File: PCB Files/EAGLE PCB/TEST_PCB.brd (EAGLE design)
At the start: 33.6 x 25.5 mm, 22 parts, among them IC1 4066D, IC2 OP-AMP

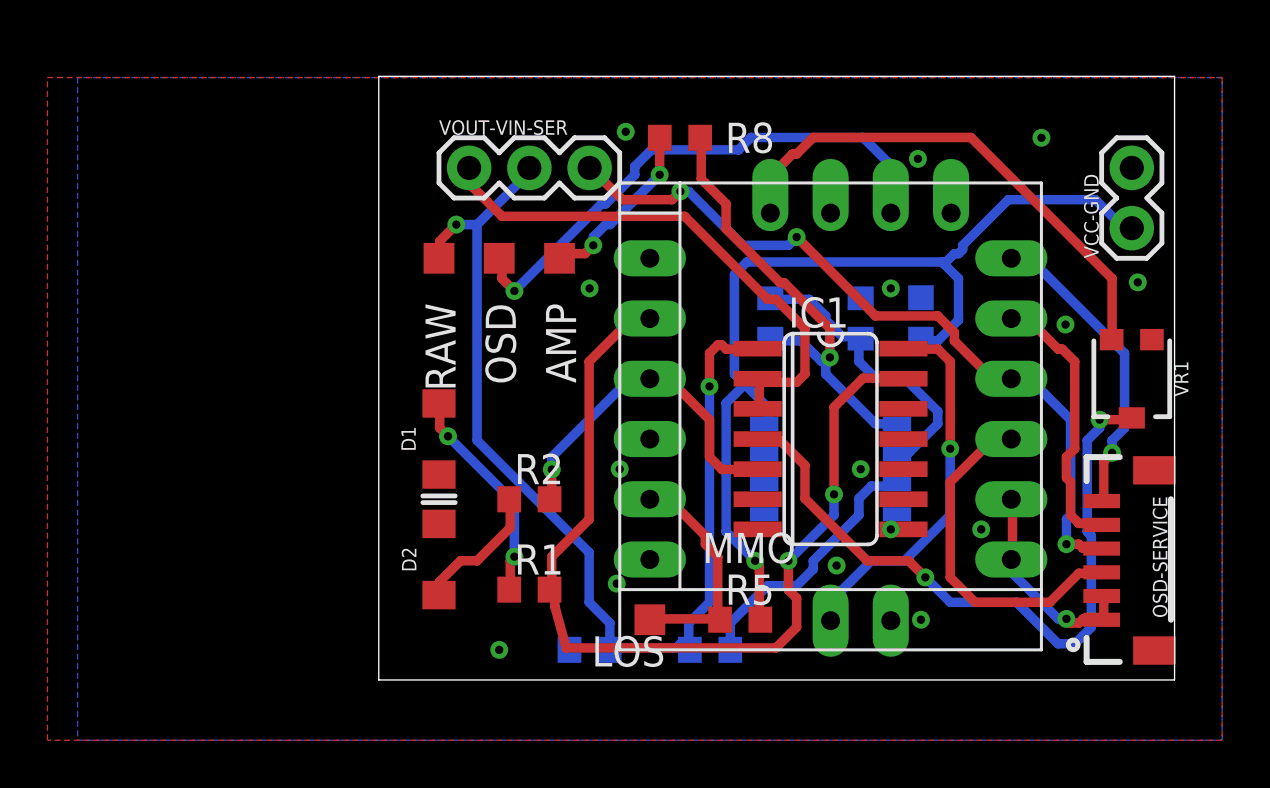
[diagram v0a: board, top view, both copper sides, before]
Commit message: Experimental PCBs
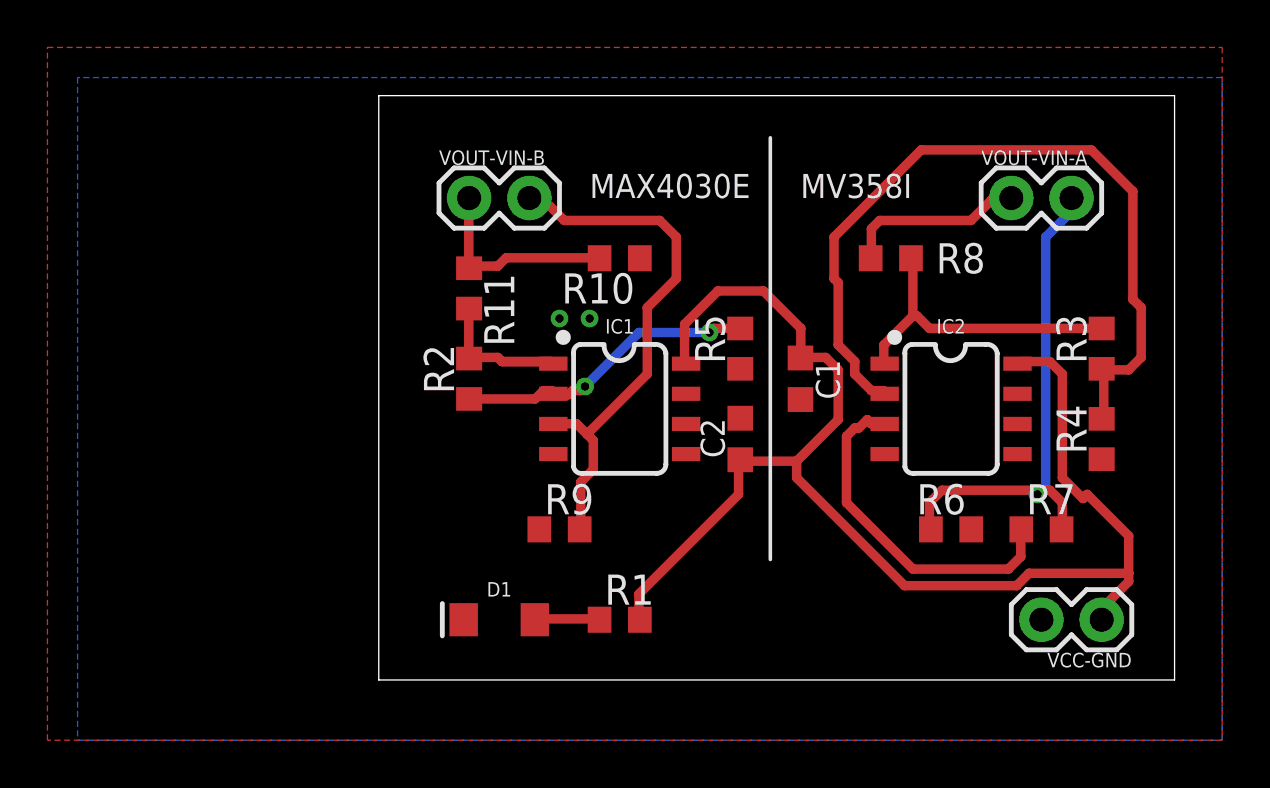
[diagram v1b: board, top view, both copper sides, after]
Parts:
- removed AMP, LOS, OSD, RAW: TPSQTP13SQ, testpad:TP13SQ
- removed D2: RED, SparkFun-LED:LED-1206
- removed MINIMOSD: MICROMINIMOSDPWR, FPVTools:MMOSDNVDVID
- removed OSD-SERVICE: EM406, SparkFun-Connectors:1X06-1MM
- removed VOUT-VIN-SER: (no value), SparkFun-Connectors:1X03
- removed VR1: 10k, SparkFun-Resistors:TRIMPOT-SMD-3MM-CLOSED
- added C2: o.1uF, rcl:C0603K
- added R10, R11, R9: 75, resistor:R0603
- added VOUT-VIN-A, VOUT-VIN-B: (no value), SparkFun-Connectors:1X02
- IC1: value 4066D -> OP-AMP; device 40xx:SO14 -> SparkFun-IC-Amplifiers:SO08
- R2: value 330 -> 200
- R5: value 1k -> 200
- moved VCC-GND 16.6 mm to (41.9, 53.3), turned to 180 degrees
- moved R6 16.1 mm to (35.6, 57.1), flipped to the top
- moved R7 14.9 mm to (39.4, 57.1), flipped to the top
- moved R3 14.0 mm to (41.9, 64.8), flipped to the top, turned to 90 degrees
- moved R5 11.4 mm to (26.7, 64.8), turned to 90 degrees
- moved R4 11.4 mm to (41.9, 61.0), flipped to the top, turned to 90 degrees
- moved R8 10.2 mm to (33.0, 68.6)
- moved IC1 8.98 mm to (21.6, 62.2)
- moved D1 8.03 mm to (16.5, 53.3), turned to 180 degrees
- moved IC2 5.68 mm to (35.6, 62.2), flipped to the top
- moved C1 5.68 mm to (29.2, 63.5), flipped to the top, turned to 270 degrees
- moved R2 5.68 mm to (15.2, 63.5), turned to 90 degrees
- moved R1 4.02 mm to (21.6, 53.3)
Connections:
- removed net 5VFTDI: MINIMOSD.VCC, OSD-SERVICE.3
- removed net AMP: AMP.TP, R8.1
- removed net BAT2: MINIMOSD.BAT2
- removed net CONTROLL_A: IC1.13, MINIMOSD.CGND, R1.2
- removed net CONTROLL_B: IC1.5, MINIMOSD.RSSI, R2.2
- removed net DTR: MINIMOSD.DTR, OSD-SERVICE.6
- removed net G: MINIMOSD.GND1, MINIMOSD.GND2, OSD-SERVICE.1, OSD-SERVICE.2
- removed net N$3: LOS.TP, MINIMOSD.BAT1, R5.1
- removed net N$6: MINIMOSD.VIDOUT, VR1.3
- removed net OSD: MINIMOSD.VIDIN, OSD.TP
- removed net OSD_OUT: IC1.4, VR1.2
- removed net RX: MINIMOSD.RX, OSD-SERVICE.4, VOUT-VIN-SER.3
- removed net TX: MINIMOSD.TX, OSD-SERVICE.5
- removed net VDD: IC1.14, MINIMOSD.IVCC
- removed net VIDEO_IN: IC1.1, R6.2, R7.2, RAW.TP, VOUT-VIN-SER.2
- removed net VIDEO_OUT: IC1.2, IC1.3, VOUT-VIN-SER.1
- removed net VSS: IC1.7
- new net 1: IC1.1, R11.2, R2.2
- new net VIDEO_IN_A: R6.2, R7.2, VOUT-VIN-A.2
- new net VIDEO_IN_B: IC1.3, R9.2, VOUT-VIN-B.2
- new net VIDEO_OUT_A: R8.1, VOUT-VIN-A.1
- new net VIDEO_OUT_B: R10.2, R11.1, VOUT-VIN-B.1
- net GND: now also C2.2, IC1.4, R10.1, R5.1, R9.1; no longer D2.C, IC1.11, IC1.8, MINIMOSD.BGND, MINIMOSD.CUR, MINIMOSD.IGND, MINIMOSD.VGND1, MINIMOSD.VGND2
- net N$1: now also IC1.2, R5.2; no longer D2.A
- net VCC: now also C2.1, IC1.8, R1.2; no longer R5.2
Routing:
- net VIDEO_IN: track 45.3 -> 0.00 mm, vias 2 -> 0
- net CONTROLL_A: track 40.3 -> 0.00 mm, vias 2 -> 0
- net RX: track 32.4 -> 0.00 mm, vias 3 -> 0
- net OSD_OUT: track 29.2 -> 0.00 mm, vias 2 -> 0
- net OSD: track 22.9 -> 0.00 mm, vias 1 -> 0
- net VIDEO_OUT: track 22.8 -> 0.00 mm
- net VIDEO_IN_B: track 0.00 -> 22.7 mm
- net N$6: track 21.7 -> 0.00 mm
- net VIDEO_IN_A: track 0.00 -> 21.7 mm, vias 0 -> 1
- net N$4: track 12.6 -> 34.0 mm
- net VCC: track 41.2 -> 57.9 mm, vias 1 -> 0
- net VDD: track 16.1 -> 0.00 mm, vias 1 -> 0
- net 5VFTDI: track 14.7 -> 0.00 mm
- net CONTROLL_B: track 14.5 -> 0.00 mm, vias 1 -> 0
- net DTR: track 13.1 -> 0.00 mm, vias 1 -> 0
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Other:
- board size 33.6 x 25.5 mm -> 33.6 x 24.6 mm
- board text added: "MAX4030E"
- board text added: "MV358I"
